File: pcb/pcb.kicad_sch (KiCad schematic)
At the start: 1 part

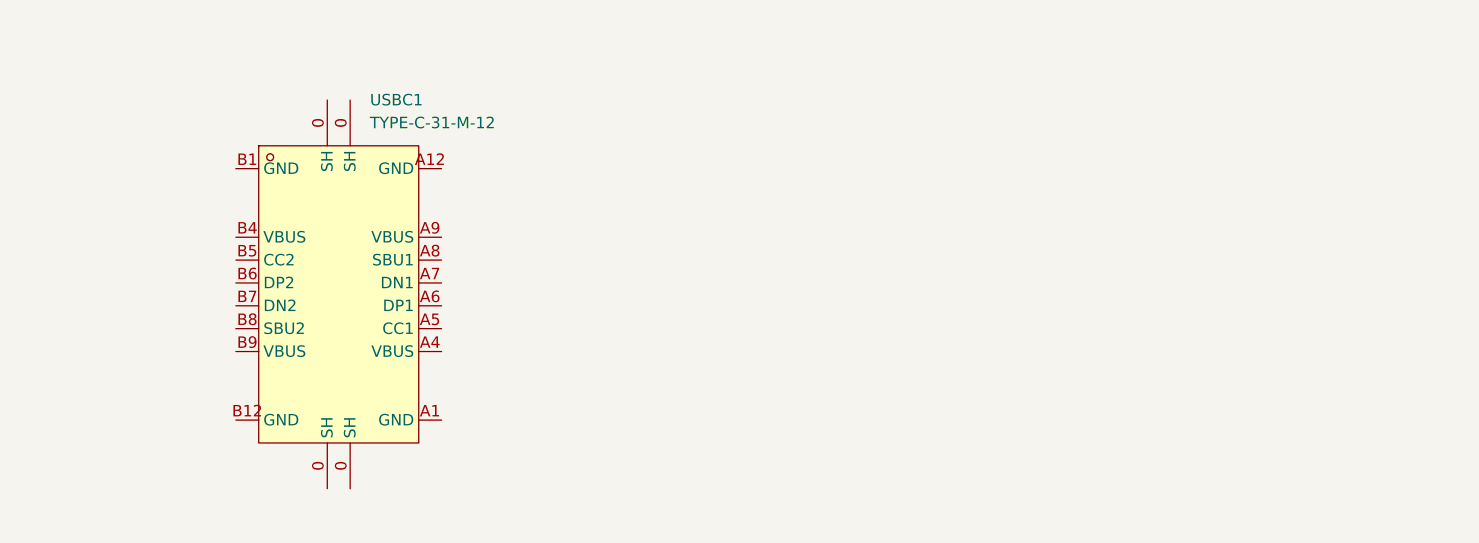
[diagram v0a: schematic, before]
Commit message: More playing with JLCPCB
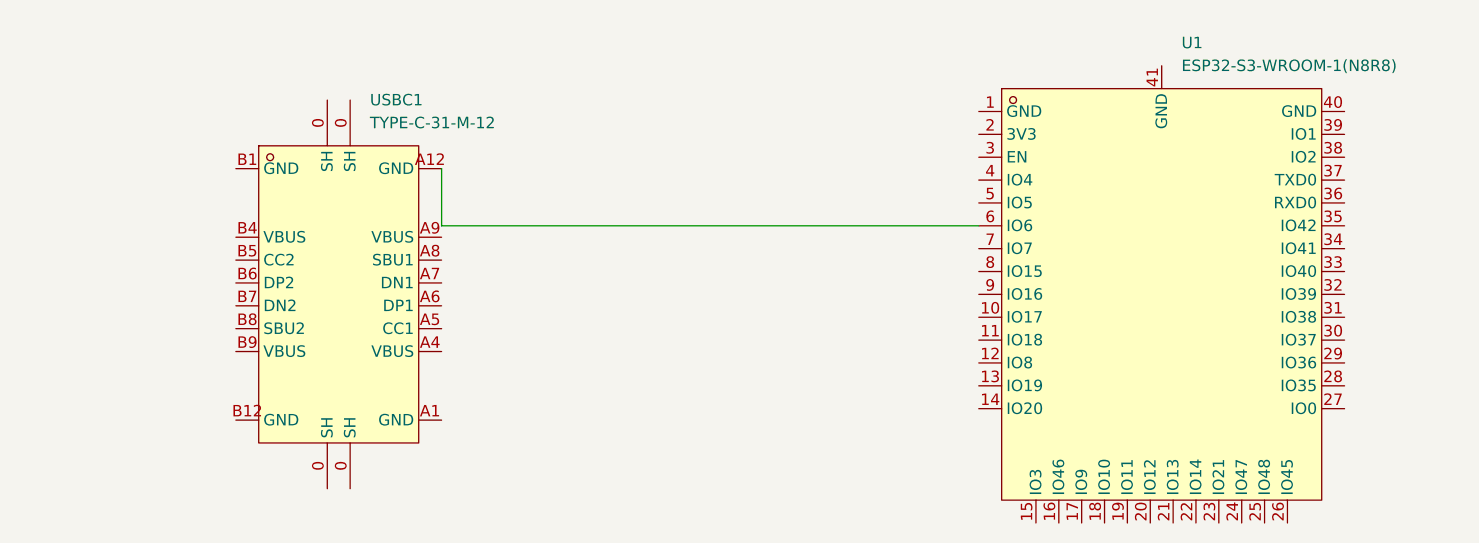
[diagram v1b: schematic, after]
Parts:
- added U1: ESP32-S3-WROOM-1(N8R8), EasyEDA:WIRELM-SMD_ESP32-S3-WROOM-1, symbol EasyEDA:ESP32-S3-WROOM-1(N8R8)
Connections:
- net at USBC1.A12 (GND): now also U1.6 (IO6)
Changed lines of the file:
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@@
 	(generator_version "8.0")
 	(paper "A4")
+	(wire
+		(pts
+			(xy 140.97 50.8) (xy 81.28 50.8)
+		)
+		(stroke
+			(width 0)
+			(type default)
+		)
+	)
+	(wire
+		(pts
+			(xy 81.28 50.8) (xy 81.28 44.45)
+		)
+		(stroke
+			(width 0)
+			(type default)
+		)
+	)
+	(symbol
+		(lib_id "EasyEDA:ESP32-S3-WROOM-1(N8R8)")
+		(at 161.29 58.42 0)
+		(unit 1)
+		(exclude_from_sim no)
+		(in_bom yes)
+		(on_board yes)
+		(dnp no)
+		(fields_autoplaced yes)
+		(property "Reference" "U1"
+			(at 163.4841 30.48 0)
+			(effects
+				(font
+					(size 1.27 1.27)
+				)
+				(justify left)
+			)
+		)
+		(property "Value" "ESP32-S3-WROOM-1(N8R8)"
+			(at 163.4841 33.02 0)
+			(effects
+				(font
+					(size 1.27 1.27)
+				)
+				(justify left)
+			)
+		)
+		(property "Footprint" "EasyEDA:WIRELM-SMD_ESP32-S3-WROOM-1"
+			(at 161.29 91.44 0)
+			(effects
+				(font
+					(size 1.27 1.27)
+				)
+				(hide yes)
+			)
+		)
+		(property "Datasheet" ""
+			(at 161.29 58.42 0)
+			(effects
+				(font
+					(size 1.27 1.27)
+				)
+				(hide yes)
+			)
+		)
+		(property "Description" ""
+			(at 161.29 58.42 0)
+			(effects
+				(font
+					(size 1.27 1.27)
+				)
+				(hide yes)
+			)
+		)
+		(property "LCSC Part" "C2913201"
+			(at 161.29 93.98 0)
+			(effects
+				(font
+					(size 1.27 1.27)
+				)
+				(hide yes)
+			)
+		)
+		(pin "14"
+		)
+		(pin "21"
+		)
+		(pin "38"
+		)
+		(pin "11"
+		)
+		(pin "1"
+		)
+		(pin "12"
+		)
+		(pin "10"
+		)
+		(pin "16"
+		)
+		(pin "39"
+		)
+		(pin "25"
+		)
+		(pin "26"
+		)
+		(pin "31"
+		)
+		(pin "6"
+		)
+		(pin "7"
+		)
+		(pin "4"
+		)
+		(pin "33"
+		)
+		(pin "15"
+		)
+		(pin "29"
+		)
+		(pin "23"
+		)
+		(pin "28"
+		)
+		(pin "32"
+		)
+		(pin "34"
+		)
+		(pin "18"
+		)
+		(pin "17"
+		)
+		(pin "24"
+		)
+		(pin "2"
+		)
+		(pin "37"
+		)
+		(pin "40"
+		)
+		(pin "19"
+		)
+		(pin "3"
+		)
+		(pin "30"
+		)
+		(pin "35"
+		)
+		(pin "20"
+		)
+		(pin "27"
+		)
+		(pin "9"
+		)
+		(pin "41"
+		)
+		(pin "5"
+		)
+		(pin "8"
+		)
+		(pin "36"
+		)
+		(pin "13"
+		)
+		(pin "22"
+		)
+		(instances
+			(project ""
+				(path "/7efcc018-2ceb-4b85-a682-18e44d24826b"
+					(reference "U1")
+					(unit 1)
+				)
+			)
+		)
+	)
 	(symbol
 		(lib_id "EasyEDA:TYPE-C-31-M-12")

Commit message: Much more work
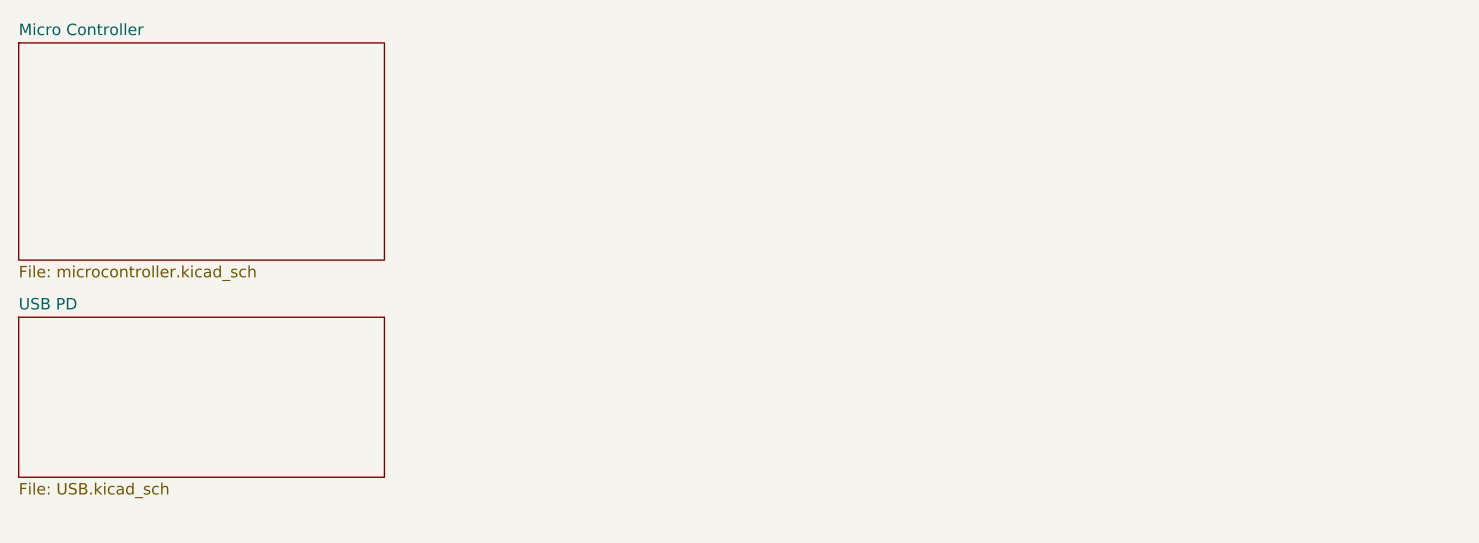
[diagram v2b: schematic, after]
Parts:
- removed U1: ESP32-S3-WROOM-1(N8R8), EasyEDA:WIRELM-SMD_ESP32-S3-WROOM-1, symbol EasyEDA:ESP32-S3-WROOM-1(N8R8)
- removed USBC1: TYPE-C-31-M-12, EasyEDA:USB-C_SMD-TYPE-C-31-M-12, symbol EasyEDA:TYPE-C-31-M-12
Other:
- added sheet Micro Controller (microcontroller.kicad_sch)
- added sheet USB PD (USB.kicad_sch)
